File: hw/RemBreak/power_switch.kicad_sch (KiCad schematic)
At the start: 33 parts, among them IC1 LTC2943IDD#TRPBF, IC2 MAX17049G+T10, Q10 BC337, Q11 BC847, Q12 Si7141DP, Q13 BC337, Q14 BC847, U2 INA219BxDCN, U6 BD4830FVE-TR

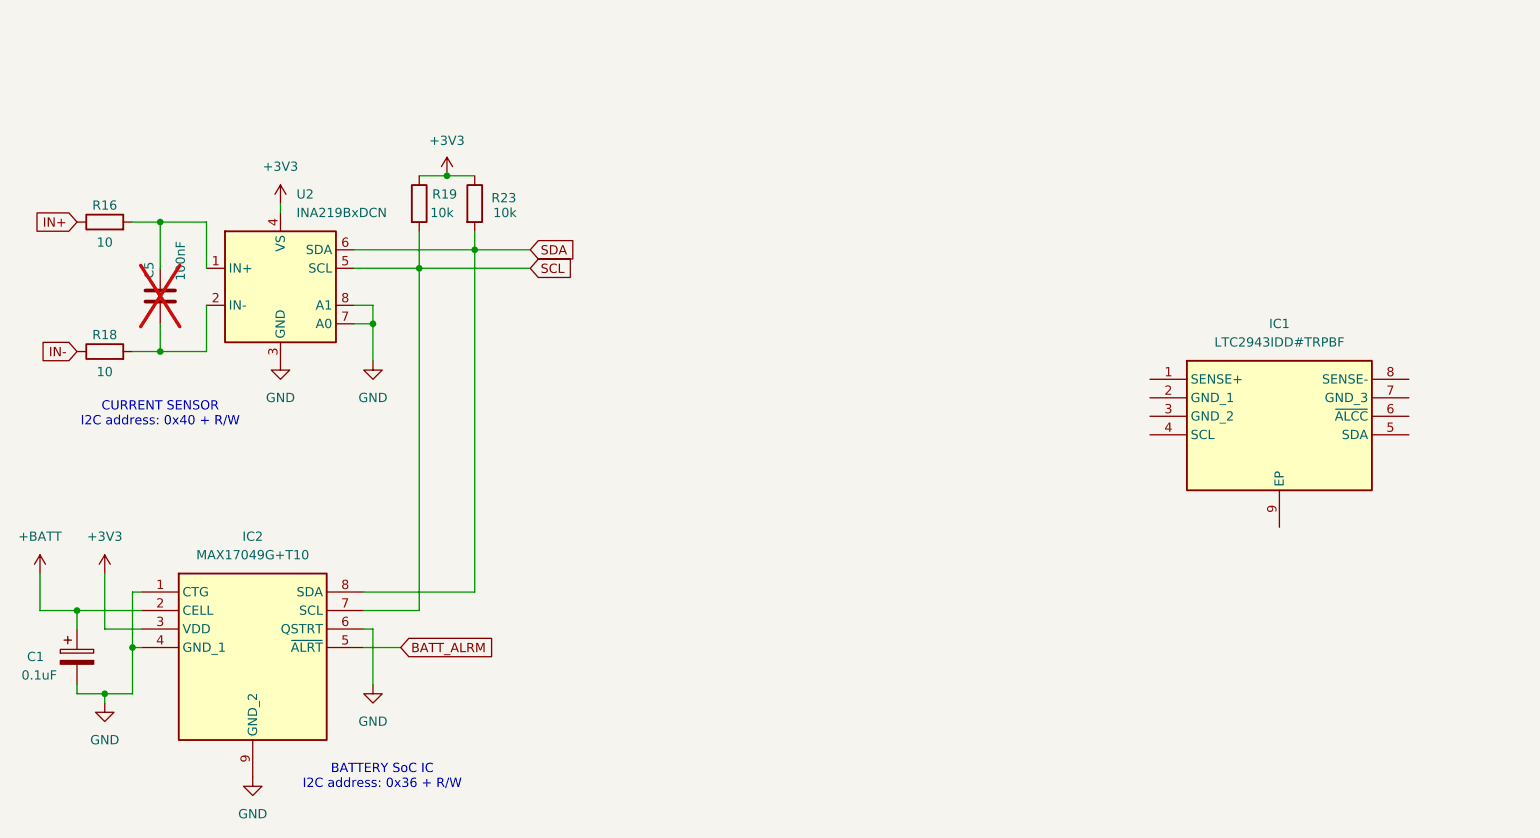
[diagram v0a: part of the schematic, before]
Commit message: reorganized subsheets
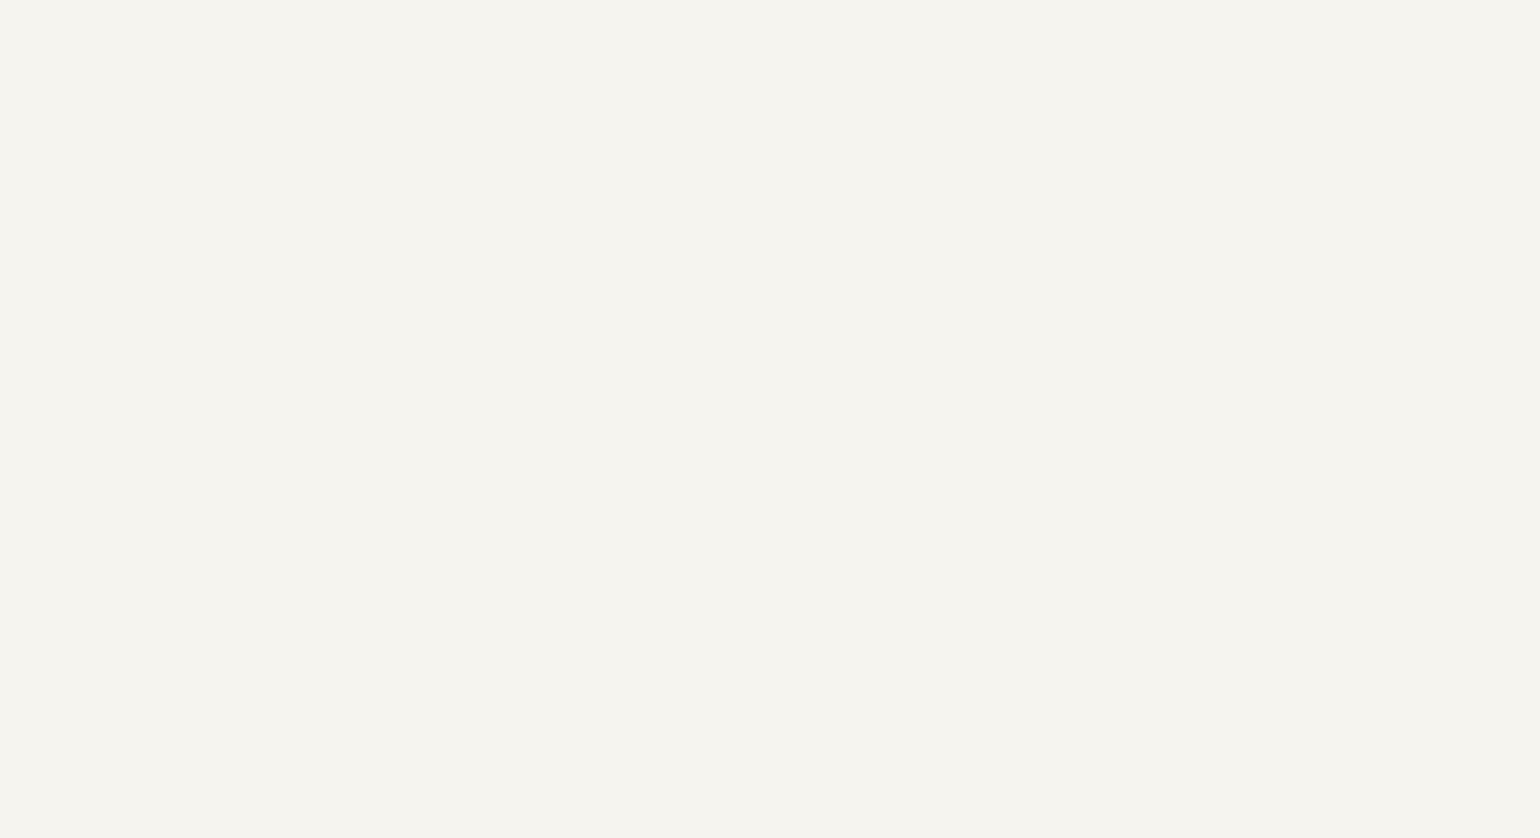
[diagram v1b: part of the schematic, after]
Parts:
- removed C1: 0.1uF, symbol Device:C_Polarized
- removed C5: 100nF, symbol Device:C
- removed IC1: LTC2943IDD#TRPBF, SON50P300X300X80-9N-D, symbol dodo-device:LTC2943IDD#TRPBF
- removed IC2: MAX17049G+T10, Package_DFN_QFN:TDFN-8-1EP_2x2mm_P0.5mm_EP0.8x1.2mm, symbol dodo-power:MAX17049G+T10
- removed R16, R18: 10, symbol Device:R
- removed R19, R23: 10k, symbol Device:R
- removed U2: INA219BxDCN, Package_TO_SOT_SMD:SOT-23-8, symbol Analog_ADC:INA219BxDCN
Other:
- note removed: "BATTERY SoC IC I2C address: 0x36 + R/W"
- note removed: "CURRENT SENSOR I2C address: 0x40 + R/W"
